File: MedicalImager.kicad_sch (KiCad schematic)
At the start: 0 parts

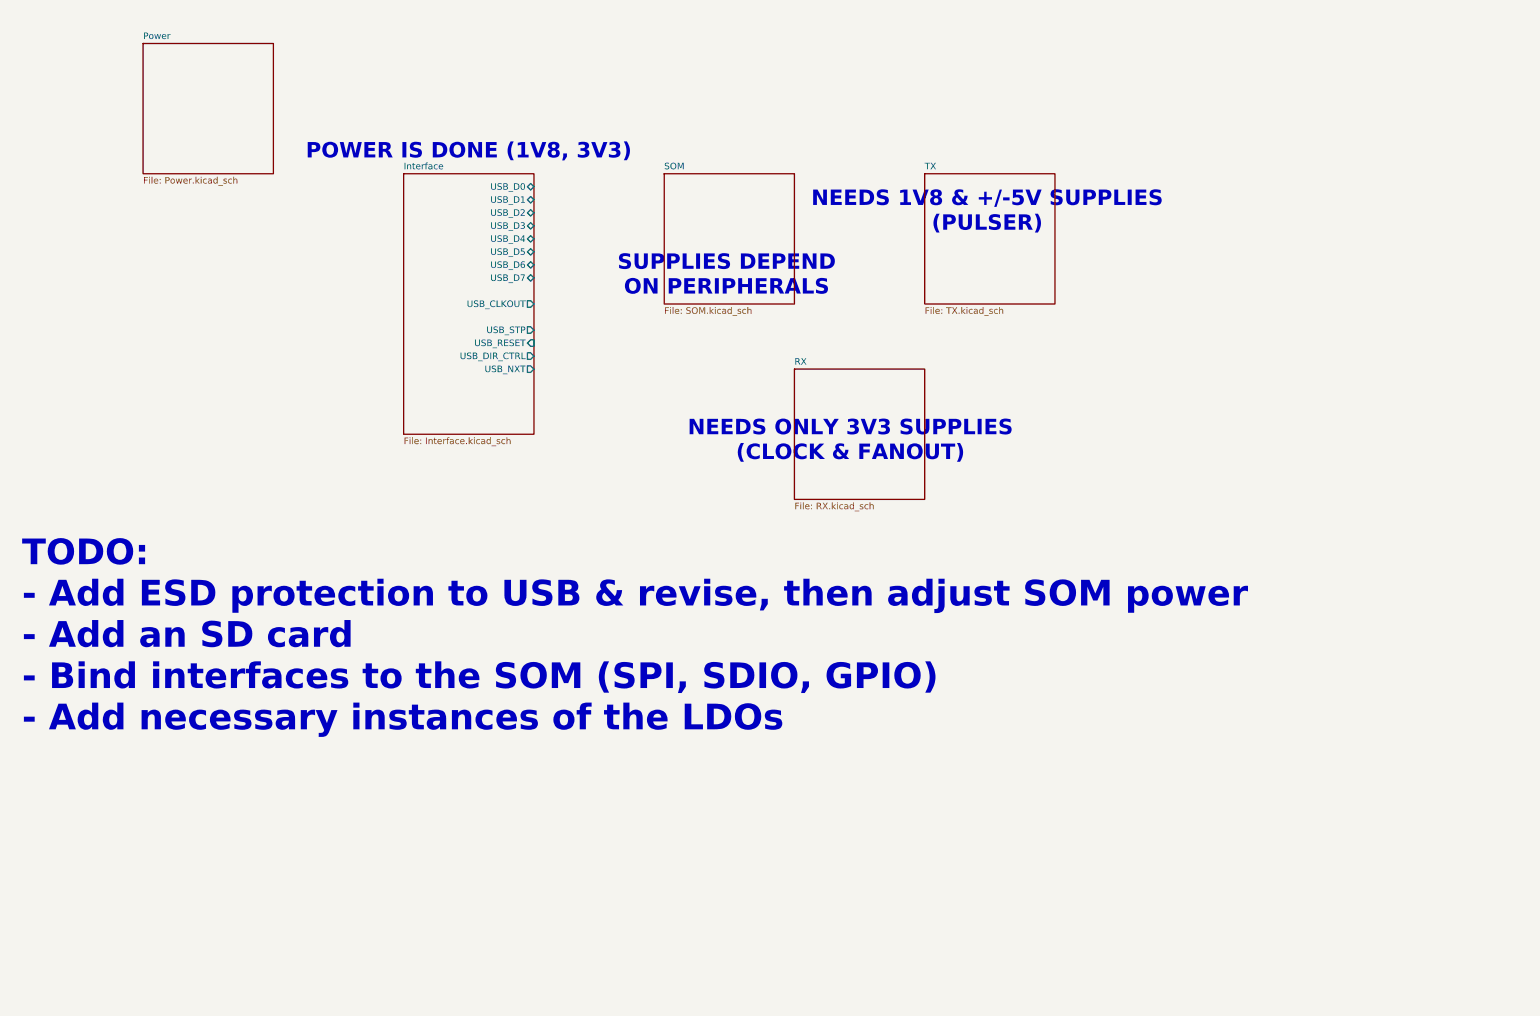
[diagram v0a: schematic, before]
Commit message: almost finished, phew! just dd +/- 5v rails, connect the SDIO & power enable pins and figure out the rest of the clocking chain
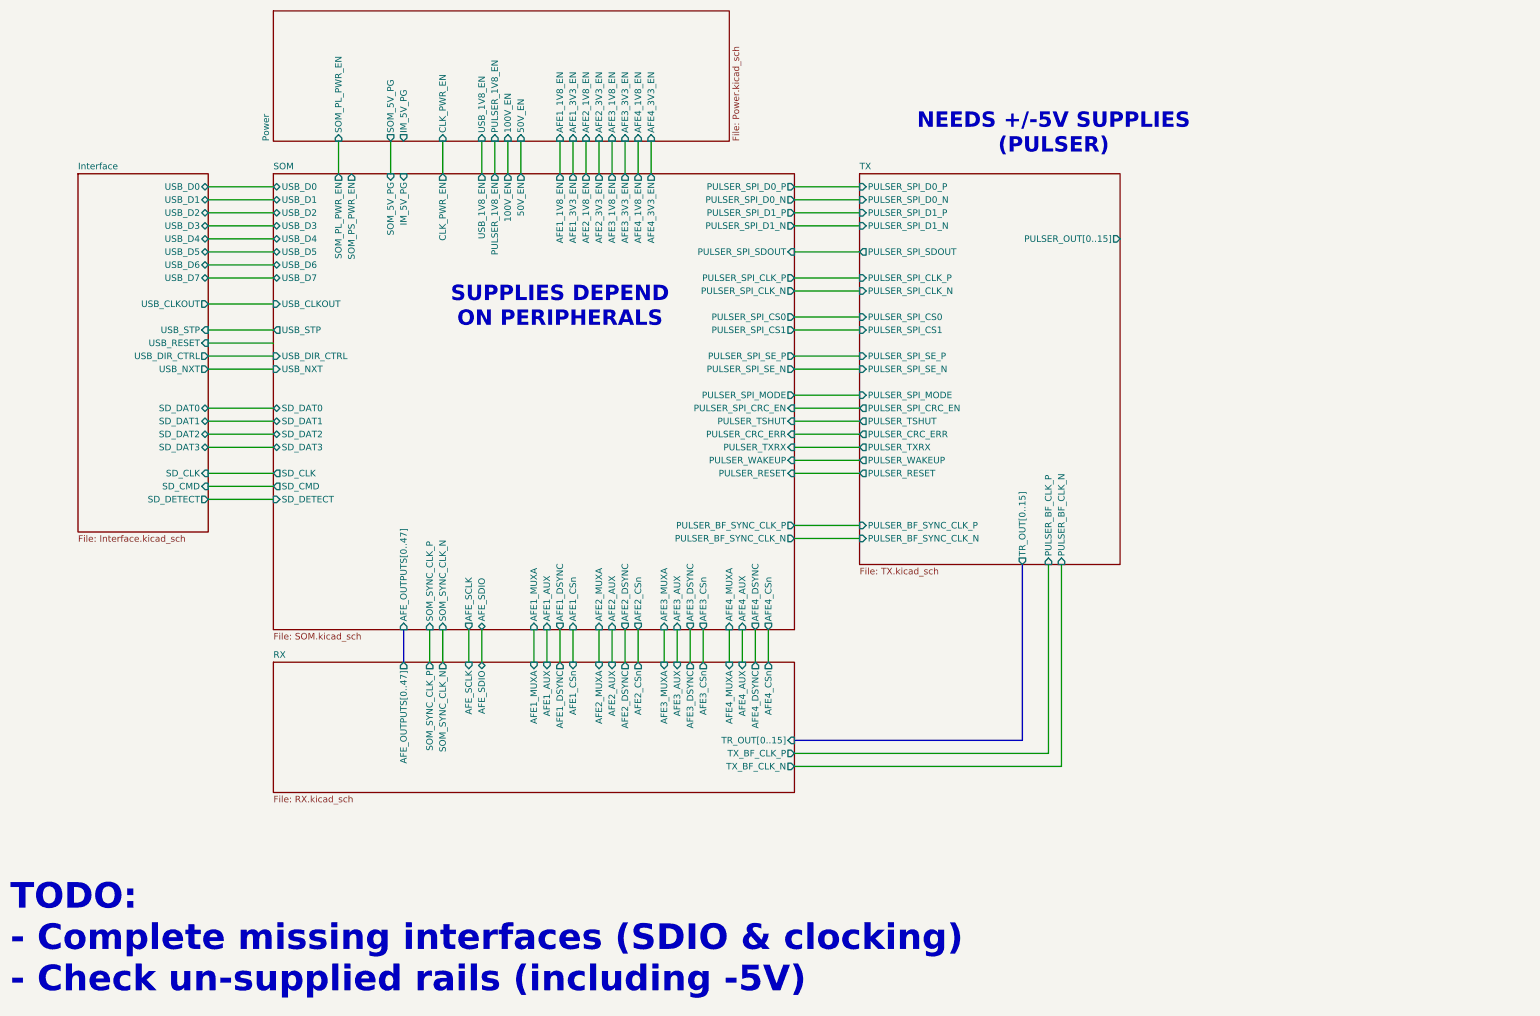
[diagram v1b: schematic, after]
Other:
- sheet Interface ports: added SD_CLK, SD_CMD, SD_DAT0, SD_DAT1, SD_DAT2, SD_DAT3, SD_DETECT; removed none
- sheet Power ports: added 100V_EN, 50V_EN, AFE1_1V8_EN, AFE1_3V3_EN, AFE2_1V8_EN, AFE2_3V3_EN, AFE3_1V8_EN, AFE3_3V3_EN, AFE4_1V8_EN, AFE4_3V3_EN, CLK_PWR_EN, IM_5V_PG, PULSER_1V8_EN, SOM_5V_PG, SOM_PL_PWR_EN, USB_1V8_EN; removed none
- sheet RX ports: added AFE1_AUX, AFE1_CSn, AFE1_DSYNC, AFE1_MUXA, AFE2_AUX, AFE2_CSn, AFE2_DSYNC, AFE2_MUXA, AFE3_AUX, AFE3_CSn, AFE3_DSYNC, AFE3_MUXA, AFE4_AUX, AFE4_CSn, AFE4_DSYNC, AFE4_MUXA, AFE_OUTPUTS[0..47], AFE_SCLK, AFE_SDIO, SOM_SYNC_CLK_N, SOM_SYNC_CLK_P, TR_OUT[0..15], TX_BF_CLK_N, TX_BF_CLK_P; removed none
- sheet SOM ports: added 100V_EN, 50V_EN, AFE1_1V8_EN, AFE1_3V3_EN, AFE1_AUX, AFE1_CSn, AFE1_DSYNC, AFE1_MUXA, AFE2_1V8_EN, AFE2_3V3_EN, AFE2_AUX, AFE2_CSn, AFE2_DSYNC, AFE2_MUXA, AFE3_1V8_EN, AFE3_3V3_EN, AFE3_AUX, AFE3_CSn, AFE3_DSYNC, AFE3_MUXA, AFE4_1V8_EN, AFE4_3V3_EN, AFE4_AUX, AFE4_CSn, AFE4_DSYNC, AFE4_MUXA, AFE_OUTPUTS[0..47], AFE_SCLK, AFE_SDIO, CLK_PWR_EN, IM_5V_PG, PULSER_1V8_EN, PULSER_BF_SYNC_CLK_N, PULSER_BF_SYNC_CLK_P, PULSER_CRC_ERR, PULSER_RESET, PULSER_SPI_CLK_N, PULSER_SPI_CLK_P, PULSER_SPI_CRC_EN, PULSER_SPI_CS0, PULSER_SPI_CS1, PULSER_SPI_D0_N, PULSER_SPI_D0_P, PULSER_SPI_D1_N, PULSER_SPI_D1_P, PULSER_SPI_MODE, PULSER_SPI_SDOUT, PULSER_SPI_SE_N, PULSER_SPI_SE_P, PULSER_TSHUT, PULSER_TXRX, PULSER_WAKEUP, SD_CLK, SD_CMD, SD_DAT0, SD_DAT1, SD_DAT2, SD_DAT3, SD_DETECT, SOM_5V_PG, SOM_PL_PWR_EN, SOM_PS_PWR_EN, SOM_SYNC_CLK_N, SOM_SYNC_CLK_P, USB_1V8_EN, USB_CLKOUT, USB_D0, USB_D1, USB_D2, USB_D3, USB_D4, USB_D5, USB_D6, USB_D7, USB_DIR_CTRL, USB_NXT, USB_STP; removed none
- sheet TX ports: added PULSER_BF_CLK_N, PULSER_BF_CLK_P, PULSER_BF_SYNC_CLK_N, PULSER_BF_SYNC_CLK_P, PULSER_CRC_ERR, PULSER_OUT[0..15], PULSER_RESET, PULSER_SPI_CLK_N, PULSER_SPI_CLK_P, PULSER_SPI_CRC_EN, PULSER_SPI_CS0, PULSER_SPI_CS1, PULSER_SPI_D0_N, PULSER_SPI_D0_P, PULSER_SPI_D1_N, PULSER_SPI_D1_P, PULSER_SPI_MODE, PULSER_SPI_SDOUT, PULSER_SPI_SE_N, PULSER_SPI_SE_P, PULSER_TSHUT, PULSER_TXRX, PULSER_WAKEUP, TR_OUT[0..15]; removed none
- note added: "NEEDS +/-5V SUPPLIES (PULSER)"
- note added: "TODO: - Complete missing interfaces (SDIO & clocking) - Check un-supplied rails (including -5V)"
- note removed: "NEEDS 1V8 & +/-5V SUPPLIES (PULSER)"
- note removed: "NEEDS ONLY 3V3 SUPPLIES (CLOCK & FANOUT)"
- note removed: "POWER IS DONE (1V8, 3V3)"
- note removed: "TODO: - Add ESD protection to USB & revise, then adjust SOM power - Add an SD card - Bind interfaces to the SOM (SPI, SDIO, GPIO) - Add necessary instances of the LDOs"
